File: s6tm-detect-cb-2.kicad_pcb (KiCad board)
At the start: 4 copper layers, 175 parts, among them J1 Conn_Coaxial, J2 Conn_01x04_Pin, J3 USB_C_Receptacle_USB2.0_14P, J4 Conn_01x04, J5 Conn_01x04, J6 USB_C_Receptacle_USB2.0_14P, J7 Conn_01x04_Pin, J8 SIM_Card_Shielded, J9 Conn_Coaxial, Q1 AO3400A, Q2 MMBT3904, Q3 MMBT3904, Q4 MMBT3904, SW1 SW_Push, SW2 SW_Push, SW3 SW_Push, SW4 SW_Push, U1 W25Q128JVS, U10 TPS6282x, U11 TPS6282x, U12 TPS259472A, U13 TPD3F303DPV, U14 SIM7080G, U15 SN74LV1T125DBV, U16 SN74LV1T125DBV, U17 SN74LV1T125DBV, U18 SN74LV1T125DBV, U19 SN74LV1T125DBV, U2 SN65HVD230, U3 PCF85263ATL, U4 MS5607, U5 ESP32-S3FH4R2, U6 HTU21, U8 VL53L0CXV0DH1, U9 NextPM, Y1 32k768, Y2 48M

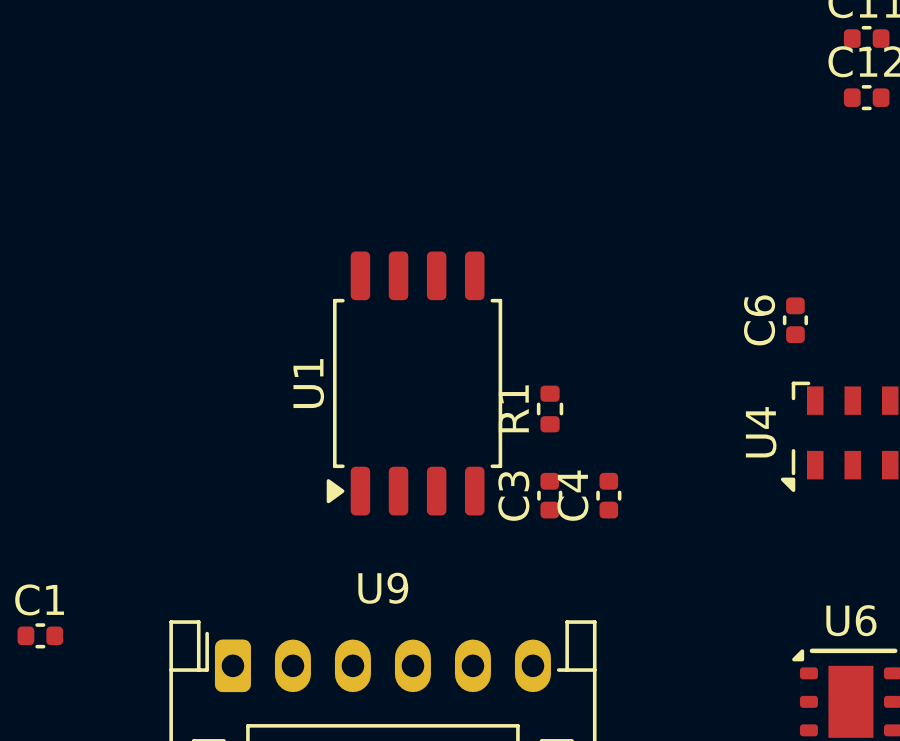
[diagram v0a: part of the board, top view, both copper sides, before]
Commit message: pcb: add flash layout
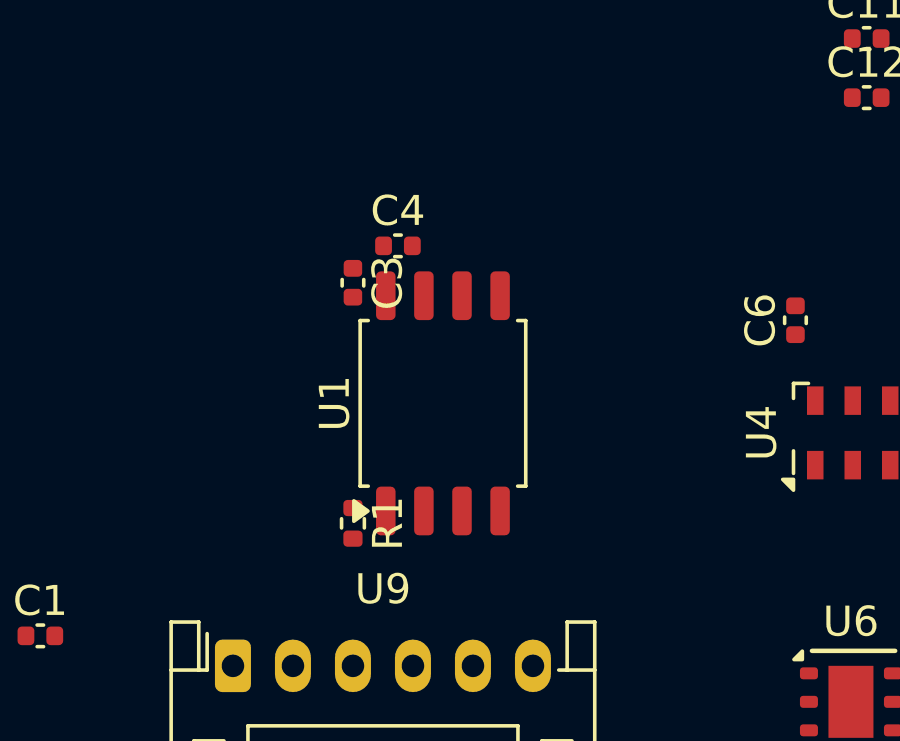
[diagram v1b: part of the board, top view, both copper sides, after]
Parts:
- moved C4 10.9 mm to (136.5, 172.2), turned to 0 degrees
- moved C3 9.66 mm to (135.0, 173.5), turned to -90 degrees
- moved R1 7.60 mm to (135.0, 181.5), turned to -90 degrees
- moved U1 1.07 mm to (138.0, 177.5)
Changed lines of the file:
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@@
 	(footprint "Package_SO:SOIC-8_5.3x5.3mm_P1.27mm"
 		(layer "F.Cu")
-		(at 137.155 176.8375 90)
+		(at 138 177.5 90)
 		(descr "SOIC, 8 Pin (JEITA/EIAJ ED-7311-19 variation 08-001-BBA and Atmel/Microchip, 208 mils width, https://www.jeita.or.jp/japanese/standard/book/ED-7311-19/#target/page_no=21, https://ww1.microchip.com/downloads/en/DeviceDoc/20005045C.pdf#page=23, https://ww1.microchip.com/downloads/en/DeviceDoc/doc2535.pdf#page=162)")
 		(tags "SOIC SO P-SOP SOP SOP-8 SO SO-8 8S2 S2AE/F K04-056 CASE-751BE SO8W 8-Pin-SOIC PSA W8-2 W8-4 W8MS-1 FPT-8P-M08")
@@
 	(footprint "Capacitor_SMD:C_0402_1005Metric"
 		(layer "F.Cu")
-		(at 143.53 180.5775 90)
+		(at 136.5 172.25)
 		(descr "Capacitor SMD 0402 (1005 Metric), square (rectangular) end terminal, IPC-7351 nominal, (Body size source: IPC-SM-782 page 76, https://www.pcb-3d.com/wordpress/wp-content/uploads/ipc-sm-782a_amendment_1_and_2.pdf)")
 		(tags "capacitor")
 		(property "Reference" "C4"
-			(at 0 -1.16 90)
+			(at 0 -1.16 0)
 			(layer "F.SilkS")
 			(effects
@@
 		)
 		(property "Value" "0u1"
-			(at 0 1.16 90)
+			(at 0 1.16 0)
 			(layer "F.Fab")
 			(effects
@@
 		)
 		(property "Datasheet" ""
-			(at 0 0 90)
+			(at 0 0 0)
 			(layer "F.Fab")
 			(hide yes)
@@
 		)
 		(property "Description" "Unpolarized capacitor"
-			(at 0 0 90)
+			(at 0 0 0)
 			(layer "F.Fab")
 			(hide yes)
@@
 		)
 		(property "KiLib_Generator" "SMD_2terminal_chip_molded"
-			(at 0 0 90)
+			(at 0 0 0)
 			(layer "F.SilkS")
 			(hide yes)
@@
 		)
 		(property "Manufacturer" "Samsung Electro-Mechanics "
-			(at 0 0 90)
+			(at 0 0 0)
 			(unlocked yes)
 			(layer "F.Fab")
@@
 		)
 		(property "Manufacturer Part Number" "CL05B104KB54PNC"
-			(at 0 0 90)
+			(at 0 0 0)
 			(unlocked yes)
 			(layer "F.Fab")
@@
 		)
 		(property "Basic" "Y"
-			(at 0 0 90)
+			(at 0 0 0)
 			(unlocked yes)
 			(layer "F.Fab")
@@
 		)
 		(property "JLCPCB Part #" "C307331"
-			(at 0 0 90)
+			(at 0 0 0)
 			(unlocked yes)
 			(layer "F.Fab")
@@
 		)
 		(property "KLC_S3.3" ""
-			(at 0 0 90)
+			(at 0 0 0)
 			(unlocked yes)
 			(layer "F.Fab")
@@
 		)
 		(property "KLC_S4.1" ""
-			(at 0 0 90)
+			(at 0 0 0)
 			(unlocked yes)
 			(layer "F.Fab")
@@
 		)
 		(fp_text user "${REFERENCE}"
-			(at 0 0 90)
+			(at 0 0 0)
 			(layer "F.Fab")
 			(effects
@@
 		)
 		(pad "1" smd roundrect
-			(at -0.48 0 90)
+			(at -0.48 0)
 			(size 0.56 0.62)
 			(layers "F.Cu" "F.Mask" "F.Paste")
@@
 		)
 		(pad "2" smd roundrect
-			(at 0.48 0 90)
+			(at 0.48 0)
 			(size 0.56 0.62)
 			(layers "F.Cu" "F.Mask" "F.Paste")
@@
 	(footprint "Capacitor_SMD:C_0402_1005Metric"
 		(layer "F.Cu")
-		(at 141.56 180.5775 90)
+		(at 135 173.48 -90)
 		(descr "Capacitor SMD 0402 (1005 Metric), square (rectangular) end terminal, IPC-7351 nominal, (Body size source: IPC-SM-782 page 76, https://www.pcb-3d.com/wordpress/wp-content/uploads/ipc-sm-782a_amendment_1_and_2.pdf)")
 		(tags "capacitor")
@@
 		)
 		(property "Manufacturer" "Samsung Electro-Mechanics "
-			(at 0 0 90)
+			(at 0 0 270)
 			(unlocked yes)
 			(layer "F.Fab")
@@
 		)
 		(property "Manufacturer Part Number" "CL05A105KA5NQNC"
-			(at 0 0 90)
+			(at 0 0 270)
 			(unlocked yes)
 			(layer "F.Fab")
@@
 		)
 		(property "Basic" "Y"
-			(at 0 0 90)
+			(at 0 0 270)
 			(unlocked yes)
 			(layer "F.Fab")
@@
 		)
 		(property "JLCPCB Part #" "C52923"
-			(at 0 0 90)
+			(at 0 0 270)
 			(unlocked yes)
 			(layer "F.Fab")
@@
 		)
 		(property "KLC_S3.3" ""
-			(at 0 0 90)
+			(at 0 0 270)
 			(unlocked yes)
 			(layer "F.Fab")
@@
 		)
 		(property "KLC_S4.1" ""
-			(at 0 0 90)
+			(at 0 0 270)
 			(unlocked yes)
 			(layer "F.Fab")
@@
 		(duplicate_pad_numbers_are_jumpers no)
 		(fp_line
-			(start -0.107836 -0.36)
-			(end 0.107836 -0.36)
+			(start -0.107836 0.36)
+			(end 0.107836 0.36)
 			(stroke
 				(width 0.12)
@@
 		)
 		(fp_line
-			(start -0.107836 0.36)
-			(end 0.107836 0.36)
+			(start -0.107836 -0.36)
+			(end 0.107836 -0.36)
 			(stroke
 				(width 0.12)
@@
 		)
 		(pad "1" smd roundrect
-			(at -0.48 0 90)
+			(at -0.48 0 270)
 			(size 0.56 0.62)
 			(layers "F.Cu" "F.Mask" "F.Paste")
@@
 		)
 		(pad "2" smd roundrect
-			(at 0.48 0 90)
+			(at 0.48 0 270)
 			(size 0.56 0.62)
 			(layers "F.Cu" "F.Mask" "F.Paste")
@@
 	(footprint "Resistor_SMD:R_0402_1005Metric"
 		(layer "F.Cu")
-		(at 141.57 177.6875 90)
+		(at 135 181.5 -90)
 		(descr "Resistor SMD 0402 (1005 Metric), square (rectangular) end terminal, IPC-7351 nominal, (Body size source: IPC-SM-782 page 72, https://www.pcb-3d.com/wordpress/wp-content/uploads/ipc-sm-782a_amendment_1_and_2.pdf)")
 		(tags "resistor")
@@
 		)
 		(property "Basic" "Y"
-			(at 0 0 90)
+			(at 0 0 270)
 			(unlocked yes)
 			(layer "F.Fab")
@@
 		)
 		(property "JLCPCB Part #" "C25744"
-			(at 0 0 90)
+			(at 0 0 270)
 			(unlocked yes)
 			(layer "F.Fab")
@@
 		)
 		(property "Manufacturer" "Uniroyal Elec"
-			(at 0 0 90)
+			(at 0 0 270)
 			(unlocked yes)
 			(layer "F.Fab")
@@
 		)
 		(property "Manufacturer Part Number" "0402WGF1002TCE"
-			(at 0 0 90)
+			(at 0 0 270)
 			(unlocked yes)
 			(layer "F.Fab")
@@
 		)
 		(property "KLC_S3.3" ""
-			(at 0 0 90)
+			(at 0 0 270)
 			(unlocked yes)
 			(layer "F.Fab")
@@
 		)
 		(property "KLC_S4.1" ""
-			(at 0 0 90)
+			(at 0 0 270)
 			(unlocked yes)
 			(layer "F.Fab")
@@
 		(duplicate_pad_numbers_are_jumpers no)
 		(fp_line
-			(start -0.153641 -0.38)
-			(end 0.153641 -0.38)
+			(start -0.153641 0.38)
+			(end 0.153641 0.38)
 			(stroke
 				(width 0.12)
@@
 		)
 		(fp_line
-			(start -0.153641 0.38)
-			(end 0.153641 0.38)
+			(start -0.153641 -0.38)
+			(end 0.153641 -0.38)
 			(stroke
 				(width 0.12)
@@
 		)
 		(pad "1" smd roundrect
-			(at -0.51 0 90)
+			(at -0.51 0 270)
 			(size 0.54 0.64)
 			(layers "F.Cu" "F.Mask" "F.Paste")
@@
 		)
 		(pad "2" smd roundrect
-			(at 0.51 0 90)
+			(at 0.51 0 270)
 			(size 0.54 0.64)
 			(layers "F.Cu" "F.Mask" "F.Paste")
